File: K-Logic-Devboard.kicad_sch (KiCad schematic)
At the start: 33 parts, among them J1 USB_C_Receptacle_USB2.0_14P, J2 Conn_01x20, J3 Conn_01x20, J4 Conn_01x03, SW1 SW_Push, U1 RP2040, U2 NCP1117-3.3_SOT223, U3 W25Q128JVS, Y1 12 Mhz

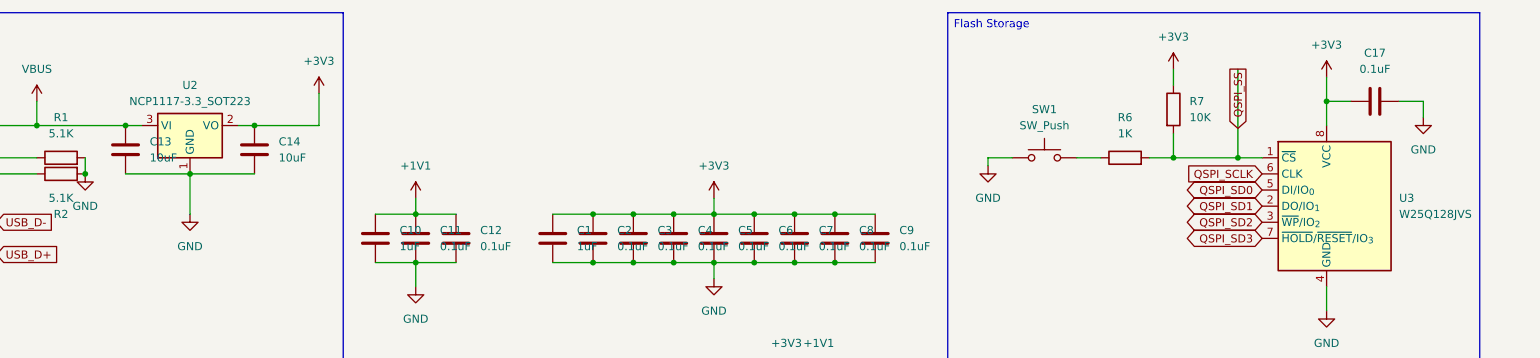
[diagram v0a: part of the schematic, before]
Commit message: third session: worked on the pcb design
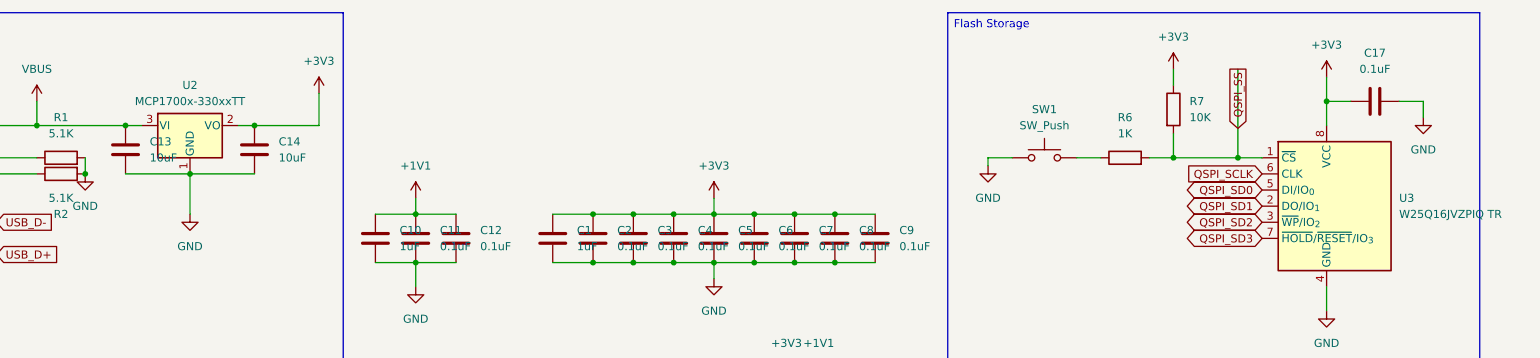
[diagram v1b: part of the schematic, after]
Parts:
- removed U2: NCP1117-3.3_SOT223, Package_TO_SOT_SMD:SOT-223-3_TabPin2, symbol Regulator_Linear:NCP1117-3.3_SOT223
- added U2: MCP1700x-330xxTT, Package_TO_SOT_SMD:SOT-23-3, symbol Regulator_Linear:MCP1700x-330xxTT
- U3: value W25Q128JVS -> W25Q16JVZPIQ TR; footprint Package_SO:SOIC-8_5.3x5.3mm_P1.27mm -> Package_SON:Winbond_USON-8-1EP_3x2mm_P0.5mm_EP0.2x1.6mm
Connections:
- net +3V3: now also U2.2 (VO)
- net GND: now also U2.1 (GND)
- net VBUS: now also U2.3 (VI)
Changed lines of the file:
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@@
 			)
 		)
-		(property "Value" "W25Q128JVS"
+		(property "Value" "W25Q16JVZPIQ TR"
 			(at 269.24 45.7199 0)
 			(effects
@@
 			)
 		)
-		(property "Footprint" "Package_SO:SOIC-8_5.3x5.3mm_P1.27mm"
+		(property "Footprint" "Package_SON:Winbond_USON-8-1EP_3x2mm_P0.5mm_EP0.2x1.6mm"
 			(at 257.81 21.59 0)
 			(effects
@@
 			)
 		)
-		(property "Datasheet" "https://www.winbond.com/resource-files/w25q128jv_dtr%20revc%2003272018%20plus.pdf"
+		(property "Datasheet" ""
 			(at 257.81 19.05 0)
 			(effects
@@
 			)
 		)
-		(property "Description" "128Mbit / 16MiB Serial Flash Memory, Standard/Dual/Quad SPI, 2.7-3.6V, SOIC-8"
+		(property "Description" ""
 			(at 257.81 16.51 0)
 			(effects
@@
 	)
 	(symbol
-		(lib_id "Regulator_Linear:NCP1117-3.3_SOT223")
-		(at 78.74 31.75 0)
-		(unit 1)
-		(exclude_from_sim no)
-		(in_bom yes)
-		(on_board yes)
-		(dnp no)
-		(fields_autoplaced yes)
-		(property "Reference" "U2"
-			(at 78.74 25.4 0)
-			(effects
-				(font
-					(size 1.27 1.27)
-				)
-			)
-		)
-		(property "Value" "NCP1117-3.3_SOT223"
-			(at 78.74 27.94 0)
-			(effects
-				(font
-					(size 1.27 1.27)
-				)
-			)
-		)
-		(property "Footprint" "Package_TO_SOT_SMD:SOT-223-3_TabPin2"
-			(at 78.74 26.67 0)
-			(effects
-				(font
-					(size 1.27 1.27)
-				)
-				(hide yes)
-			)
-		)
-		(property "Datasheet" "http://www.onsemi.com/pub_link/Collateral/NCP1117-D.PDF"
-			(at 81.28 38.1 0)
-			(effects
-				(font
-					(size 1.27 1.27)
-				)
-				(hide yes)
-			)
-		)
-		(property "Description" "1A Low drop-out regulator, Fixed Output 3.3V, SOT-223"
-			(at 78.74 31.75 0)
-			(effects
-				(font
-					(size 1.27 1.27)
-				)
-				(hide yes)
-			)
-		)
-		(pin "3"
-		)
-		(pin "1"
-		)
-		(pin "2"
-		)
-		(instances
-			(project ""
-				(path "/73a164d0-d5be-4090-91fb-c8d308b8985d"
-					(reference "U2")
-					(unit 1)
-				)
-			)
-		)
-	)
-	(symbol
 		(lib_id "power:+3V3")
 		(at 99.06 26.67 0)
@@
 					(unit 1)
 				)
+			)
+		)
+	)
+	(symbol
+		(lib_id "Regulator_Linear:MCP1700x-330xxTT")
+		(at 78.74 31.75 0)
+		(unit 1)
+		(exclude_from_sim no)
+		(in_bom yes)
+		(on_board yes)
+		(dnp no)
+		(fields_autoplaced yes)
+		(property "Reference" "U2"
+			(at 78.74 25.4 0)
+			(effects
+				(font
+					(size 1.27 1.27)
+				)
+			)
+		)
+		(property "Value" "MCP1700x-330xxTT"
+			(at 78.74 27.94 0)
+			(effects
+				(font
+					(size 1.27 1.27)
+				)
+			)
+		)
+		(property "Footprint" "Package_TO_SOT_SMD:SOT-23-3"
+			(at 78.74 26.035 0)
+			(effects
+				(font
+					(size 1.27 1.27)
+				)
+				(hide yes)
+			)
+		)
+		(property "Datasheet" "http://ww1.microchip.com/downloads/en/DeviceDoc/20001826D.pdf"
+			(at 78.74 31.75 0)
+			(effects
+				(font
+					(size 1.27 1.27)
+				)
+				(hide yes)
+			)
+		)
+		(property "Description" "250mA Low Quiscent Current LDO, 3.3V output, SOT-23"
+			(at 78.74 31.75 0)
+			(effects
+				(font
+					(size 1.27 1.27)
+				)
+				(hide yes)
+			)
+		)
+		(pin "3"
+		)
+		(pin "2"
+		)
+		(pin "1"
+		)
+		(instances
+			(project ""
+				(path "/73a164d0-d5be-4090-91fb-c8d308b8985d"
+					(reference "U2")
+					(unit 1)
+				)
